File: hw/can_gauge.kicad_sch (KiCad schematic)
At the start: 31 parts, among them J1 Gauge 1, J2 Gauge 2, J3 Gauge 3, J4 Gauge 4, J5 Gauge 5, J6 Gauge 6, J7 Power & CAN, J8 USB_B, U1 PIC16F1459-IP, U4 74HC595, U5 74HC595, U6 74HC595, U7 ULN2804A, U8 ULN2804A, U9 ULN2804A

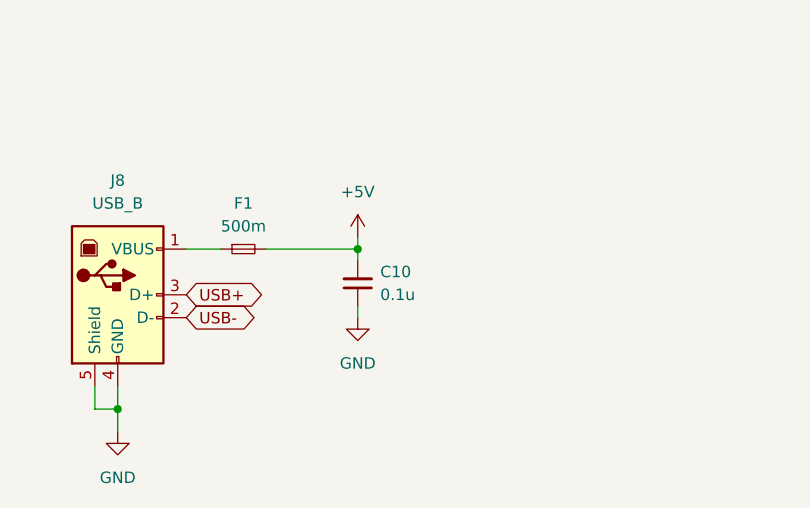
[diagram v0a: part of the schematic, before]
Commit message: hw: smd caps
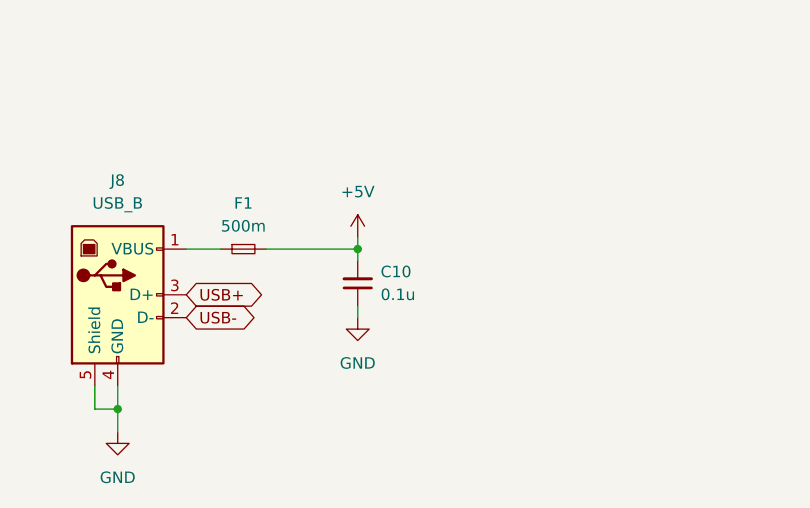
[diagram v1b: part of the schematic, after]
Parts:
- C10, C4, C5, C6, C7, C8, C9: footprint Capacitor_THT:C_Rect_L4.0mm_W2.5mm_P2.50mm -> Capacitor_SMD:C_0402_1005Metric; Digikey https://www.digikey.ca/en/products/detail/tdk-corporation/F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 -> https://www.digikey.ca/en/products/detail/murata-electronic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
- Vreg1: Digikey (none) -> https://www.digikey.ca/en/products/detail/texas-instruments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
